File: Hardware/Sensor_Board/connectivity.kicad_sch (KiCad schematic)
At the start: 19 parts, among them J501 RJ45_Input, J502 RJ45_Output, SW501 Slide Switch, U301 ICE40UL1K-CM36AI, U501 TPD4E02B04, U502 TPD4E02B04, U503 TPD4E02B04, U504 TPD4E02B04, U505 CBTU02044

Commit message: Finished final PCB checks before manufacturing and uploaded the fabrication files
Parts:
- U501, U502, U503, U504: footprint Package_SON:USON-10_2.5x1.0mm_P0.5mm -> Custom_VoxLink_Footprints:USON-10_2.5x1.0mm_P0.5mm__Reduced_Paste
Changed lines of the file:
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@@
 			)
 		)
-		(property "Footprint" "Package_SON:USON-10_2.5x1.0mm_P0.5mm"
+		(property "Footprint" "Custom_VoxLink_Footprints:USON-10_2.5x1.0mm_P0.5mm__Reduced_Paste"
 			(at 67.31 105.41 0)
 			(effects
@@
 			)
 		)
-		(property "Footprint" "Package_SON:USON-10_2.5x1.0mm_P0.5mm"
+		(property "Footprint" "Custom_VoxLink_Footprints:USON-10_2.5x1.0mm_P0.5mm__Reduced_Paste"
 			(at 226.06 97.79 0)
 			(effects
@@
 			)
 		)
-		(property "Footprint" "Package_SON:USON-10_2.5x1.0mm_P0.5mm"
+		(property "Footprint" "Custom_VoxLink_Footprints:USON-10_2.5x1.0mm_P0.5mm__Reduced_Paste"
 			(at 67.31 68.58 0)
 			(effects
@@
 			)
 		)
-		(property "Footprint" "Package_SON:USON-10_2.5x1.0mm_P0.5mm"
+		(property "Footprint" "Custom_VoxLink_Footprints:USON-10_2.5x1.0mm_P0.5mm__Reduced_Paste"
 			(at 226.06 67.31 0)
 			(effects

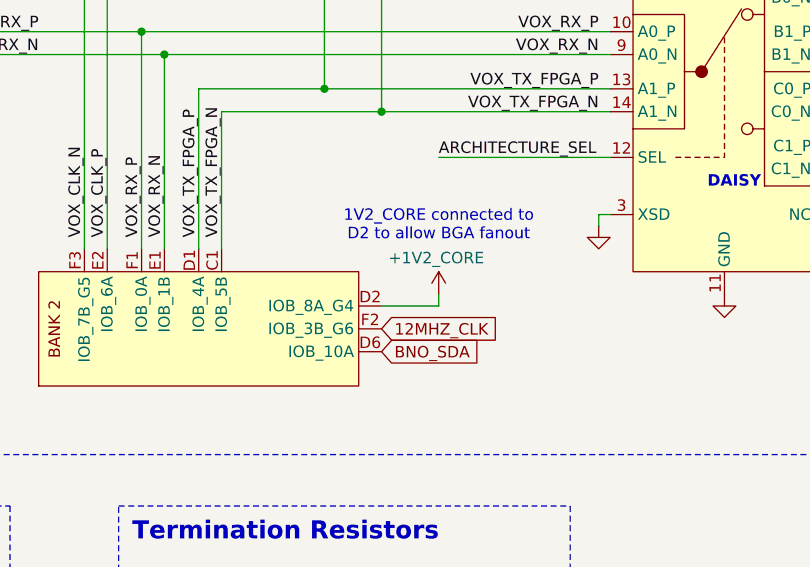
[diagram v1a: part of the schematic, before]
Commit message: Updated documentation and finished first iteration of PCB rework based on manufacturer feedback.
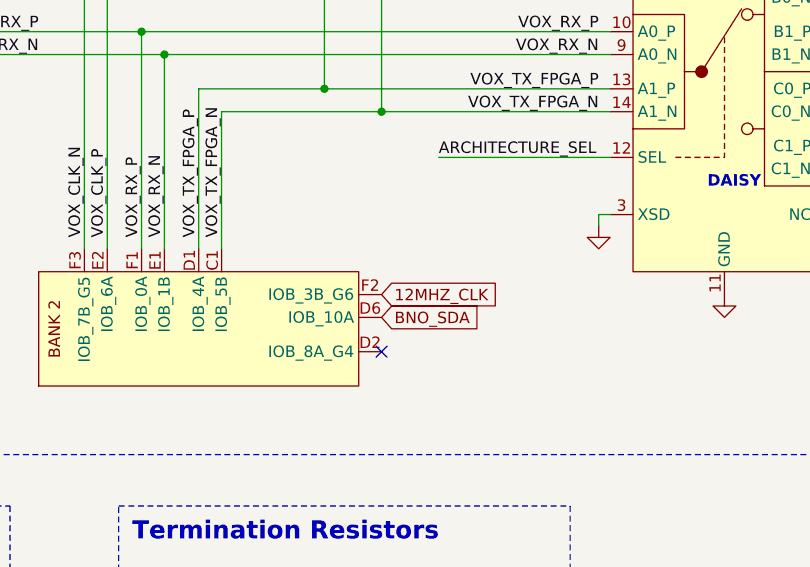
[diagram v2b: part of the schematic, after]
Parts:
- U301: footprint Custom_VoxLink_Footprints:ICE40UL1K_UCBGA-36 -> Package_BGA:UCBGA-36_2.5x2.5mm_Layout6x6_P0.4mm
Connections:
- net +1V2_CORE: no longer names the net of U301.D2 (IOB_8A_G4)
- no-connect marks 9 -> 10
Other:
- note removed: "1V2_CORE connected to D2 to allow BGA fanout"
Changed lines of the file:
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@@
 		)
 	)
-	(text "1V2_CORE connected to\nD2 to allow BGA fanout"
-		(exclude_from_sim no)
-		(at 130.81 119.38 0)
-		(effects
-			(font
-				(size 1.27 1.27)
-				(color 255 0 0 1)
-			)
-		)
-	)
 	(text "BUS"
 		(exclude_from_sim no)
@@
 	)
 	(no_connect
+		(at 124.46 133.35)
+	)
+	(no_connect
 		(at 233.68 105.41)
 	)
@@
 	(wire
 		(pts
-			(xy 130.81 128.27) (xy 130.81 127)
-		)
-		(stroke
-			(width 0)
-			(type default)
-		)
-	)
-	(wire
-		(pts
 			(xy 175.26 104.14) (xy 189.23 104.14)
 		)
@@
 	(wire
 		(pts
-			(xy 124.46 128.27) (xy 130.81 128.27)
-		)
-		(stroke
-			(width 0)
-			(type default)
-		)
-	)
-	(wire
-		(pts
 			(xy 233.68 63.5) (xy 256.54 63.5)
 		)
@@
 	(global_label "12MHZ_CLK"
 		(shape input)
-		(at 124.46 130.81 0)
+		(at 124.46 127 0)
 		(fields_autoplaced yes)
 		(effects
@@
 		)
 		(property "Intersheetrefs" "${INTERSHEET_REFS}"
-			(at 138.3913 130.81 0)
+			(at 138.3913 127 0)
 			(effects
 				(font
@@
 	(global_label "BNO_SDA"
 		(shape input)
-		(at 124.46 133.35 0)
+		(at 124.46 129.54 0)
 		(fields_autoplaced yes)
 		(effects
@@
 		)
 		(property "Intersheetrefs" "${INTERSHEET_REFS}"
-			(at 135.9119 133.35 0)
+			(at 135.9119 129.54 0)
 			(effects
 				(font
@@
 	)
 	(symbol
-		(lib_id "power:+3.3VA")
-		(at 130.81 127 0)
-		(unit 1)
-		(exclude_from_sim no)
-		(in_bom yes)
-		(on_board yes)
-		(dnp no)
-		(property "Reference" "#PWR0132"
-			(at 130.81 130.81 0)
-			(effects
-				(font
-					(size 1.27 1.27)
-				)
-				(hide yes)
-			)
-		)
-		(property "Value" "+1V2_CORE"
-			(at 125.222 122.936 0)
-			(effects
-				(font
-					(size 1.27 1.27)
-				)
-				(justify left)
-			)
-		)
-		(property "Footprint" ""
-			(at 130.81 127 0)
-			(effects
-				(font
-					(size 1.27 1.27)
-				)
-				(hide yes)
-			)
-		)
-		(property "Datasheet" ""
-			(at 130.81 127 0)
-			(effects
-				(font
-					(size 1.27 1.27)
-				)
-				(hide yes)
-			)
-		)
-		(property "Description" ""
-			(at 130.81 127 0)
-			(effects
-				(font
-					(size 1.27 1.27)
-				)
-			)
-		)
-		(pin "1"
-		)
-		(instances
-			(project "VoxSense"
-				(path "/ded7c4da-7d9f-418d-838f-f5efc7d9c9cb/68ca1e05-bb71-451f-9769-47c16f9dd6da"
-					(reference "#PWR0132")
-					(unit 1)
-				)
-			)
-		)
-	)
-	(symbol
 		(lib_id "power:GND")
 		(at 74.93 67.31 0)
@@
 			)
 		)
-		(property "Footprint" "Custom_VoxLink_Footprints:ICE40UL1K_UCBGA-36"
+		(property "Footprint" "Package_BGA:UCBGA-36_2.5x2.5mm_Layout6x6_P0.4mm"
 			(at 101.6 130.81 0)
 			(effects
